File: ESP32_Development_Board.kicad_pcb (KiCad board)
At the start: 4 copper layers, 70 x 20.3 mm, 47 parts, among them J1 Conn_01x17_Pin, J2 Conn_01x17_Pin, J3 Conn_01x03_Pin, J4 USB_B_Micro, J5 Conn_01x02_Pin, Q1 NPN, Q2 NPN, Q3 Q_NMOS_GDS, Q4 Q_NMOS_GDS, SW1 SW_Push, SW2 SW_Push, U1 ESP32-WROOM-32E, U2 CP2102N-Axx-xQFN28, U3 AMS1117-3.3

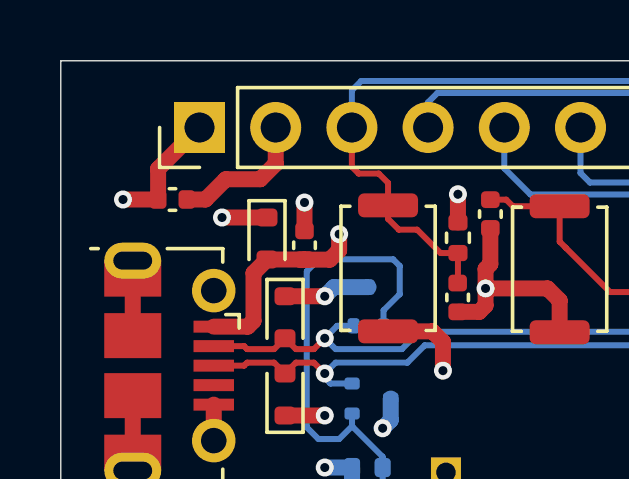
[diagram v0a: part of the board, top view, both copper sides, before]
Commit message: Commit at 2025-08-28 21:00:00
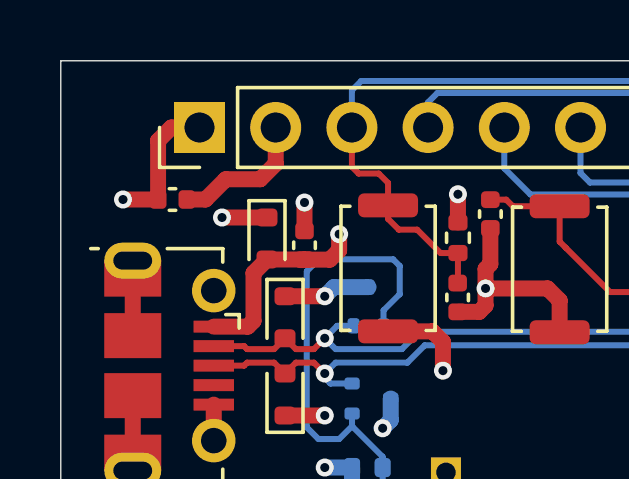
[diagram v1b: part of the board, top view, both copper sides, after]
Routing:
- net GND: track 57.1 -> 57.7 mm
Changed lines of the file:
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@@
+	)
+	(segment
+		(start 111.345 88.765)
+		(end 111.785 88.325)
+		(width 0.5334)
+		(layer "F.Cu")
+		(net 1)
 	)
 	(segment
@@
 	)
 	(segment
+		(start 111.785 88.325)
+		(end 112.725 88.325)
+		(width 0.5334)
+		(layer "F.Cu")
+		(net 1)
+	)
+	(segment
 		(start 140.33 96.95)
 		(end 139.83 96.45)
@@
 	)
 	(segment
-		(start 111.345 89.705)
-		(end 112.725 88.325)
-		(width 0.5334)
-		(layer "F.Cu")
-		(net 1)
-	)
-	(segment
 		(start 156.57 88.28)
 		(end 156.57 87.61)
@@
 	)
 	(segment
-		(start 111.345 90.725)
-		(end 111.345 89.705)
-		(width 0.5334)
-		(layer "F.Cu")
-		(net 1)
-	)
-	(segment
 		(start 124.33 93.69)
 		(end 124.73 94.09)
@@
 		(layer "F.Cu")
 		(net 1)
+	)
+	(segment
+		(start 111.345 90.725)
+		(end 111.345 88.765)
+		(width 0.5334)
+		(layer "F.Cu")
+		(net 1)
